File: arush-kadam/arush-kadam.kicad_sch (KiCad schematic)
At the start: 8 parts, among them IC1 AP63301WU-7

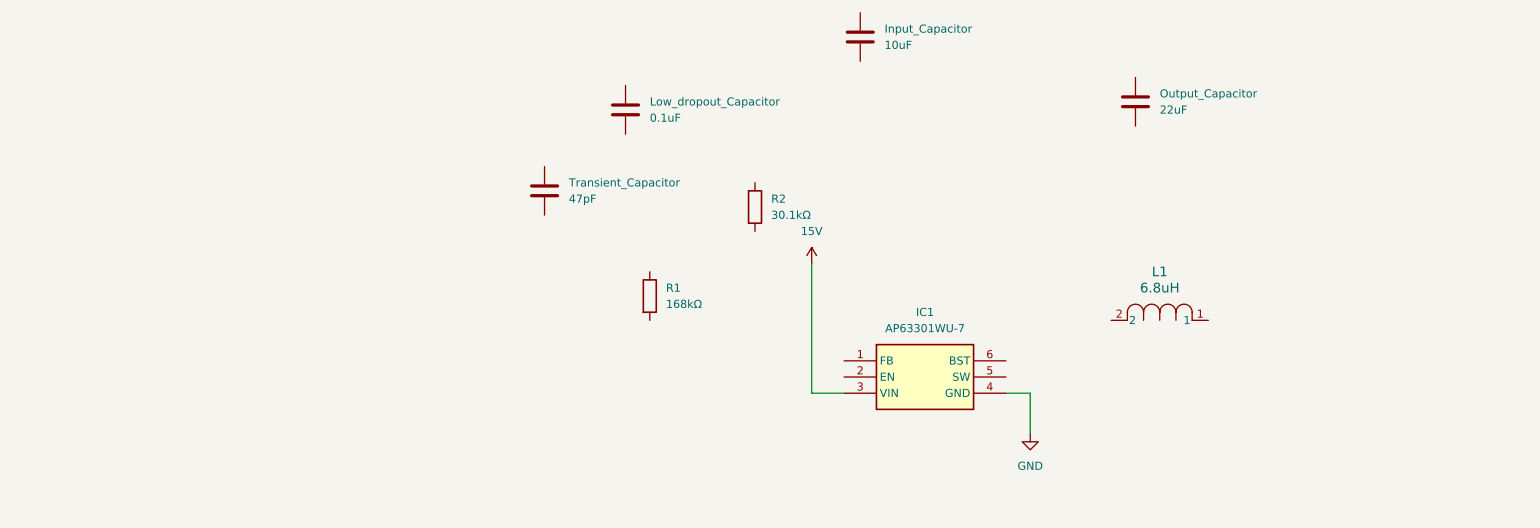
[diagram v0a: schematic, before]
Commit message: Finished wiring schematic
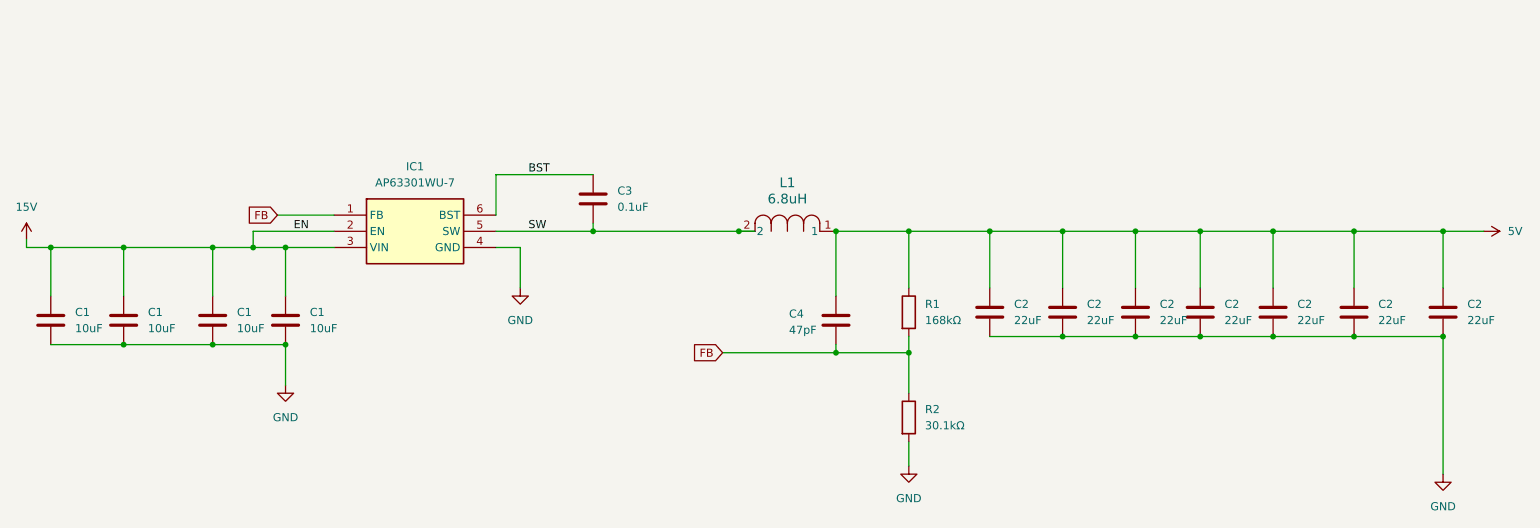
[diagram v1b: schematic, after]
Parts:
- removed Input_Capacitor: 10uF, Capacitor_SMD:C_0805_2012Metric, symbol Device:C
- removed Low_dropout_Capacitor: 0.1uF, Capacitor_SMD:C_0603_1608Metric_Pad1.05x0.95mm_HandSolder, symbol Device:C
- removed Output_Capacitor: 22uF, Capacitor_SMD:C_0805_2012Metric, symbol Device:C
- removed Transient_Capacitor: 47pF, Capacitor_SMD:C_0603_1608Metric_Pad1.05x0.95mm_HandSolder, symbol Device:C
- added C1 (x4): 10uF, Capacitor_SMD:C_0805_2012Metric, symbol Device:C
- added C2 (x7): 22uF, Capacitor_SMD:C_0805_2012Metric, symbol Device:C
- added C3: 0.1uF, Capacitor_SMD:C_0603_1608Metric_Pad1.05x0.95mm_HandSolder, symbol Device:C
- added C4: 47pF, Capacitor_SMD:C_0603_1608Metric_Pad1.05x0.95mm_HandSolder, symbol Device:C
- IC1: Digikey Part Number (none) -> 31-AP63301WU-7CT-ND; Digikey URL (none) -> https://www.digikey.com/en/products/detail/diodes-incorpora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
- L1: Digikey Part Number (none) -> SRN8040TA-6R8MCT-ND; Digikey URL (none) -> https://www.digikey.com/en/products/detail/bourns-inc/SRN80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; Manufacturer (none) -> Bourns Inc.
- R1: Digikey Part Number (none) -> 311-158KHRCT-ND; Digikey URL (none) -> https://www.digikey.com/en/products/detail/yageo/RC0603FR-0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; Manufacturer (none) -> YAGEO
- R2: Digikey Part Number (none) -> 311-30.1KHRCT-ND; Digikey URL (none) -> https://www.digikey.com/en/products/detail/yageo/RC0603FR-0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; Manufacturer (none) -> YAGEO
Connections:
- net 15V: now also IC1.2 (EN), C1.1, C1.1, C1.1, C1.1
- net GND: now also R2.2, C1.2, C1.2, C1.2, C1.2, C2.2, C2.2, C2.2, C2.2, C2.2, C2.2, C2.2
- net 5V: now reaches R1.1
- net 5V: now also L1.1, C2.1, C2.1, C2.1, C2.1, C2.1, C2.1, C2.1, C4.1
- net FB: now reaches R1.2
- net FB: now also IC1.1 (FB), R2.1, C4.2
- net SW: now reaches IC1.5 (SW)
- net SW: now also L1.2, C3.2
- net BST: now reaches IC1.6 (BST)
- net BST: now also C3.1
